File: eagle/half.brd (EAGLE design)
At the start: 138.2 x 89.8 mm, 120 parts, among them J10 AUDIO_JACK_TRRSSMD_RA, J3 AUDIO_JACK_TRRSSMD_RA, J5 AUDIO_JACK_TRRSSMD_RA, J7 AUDIO_JACK_TRRSSMD_RA, J8 AUDIO_JACK_TRRSSMD_RA, J9 AUDIO_JACK_TRRSSMD_RA

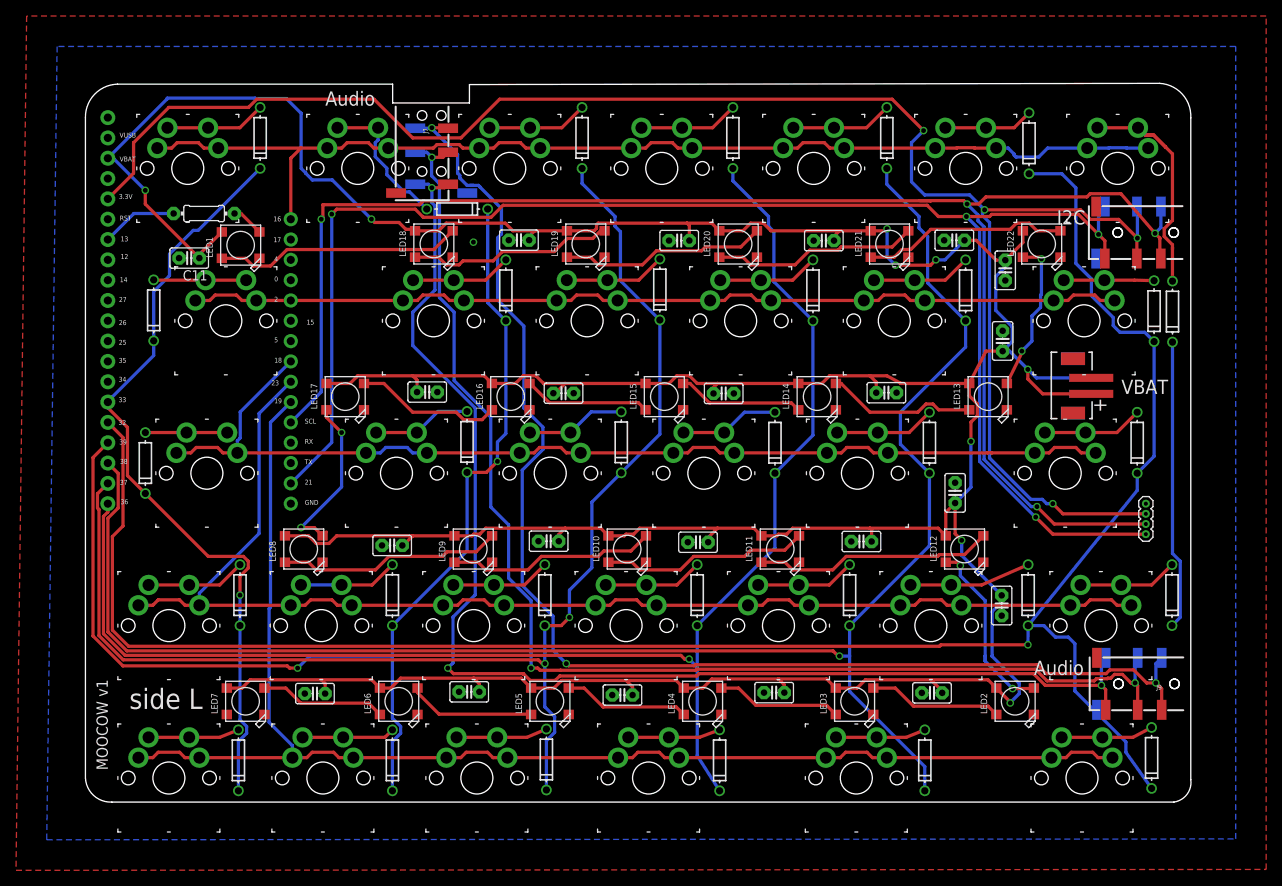
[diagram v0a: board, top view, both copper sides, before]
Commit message: updated PCB
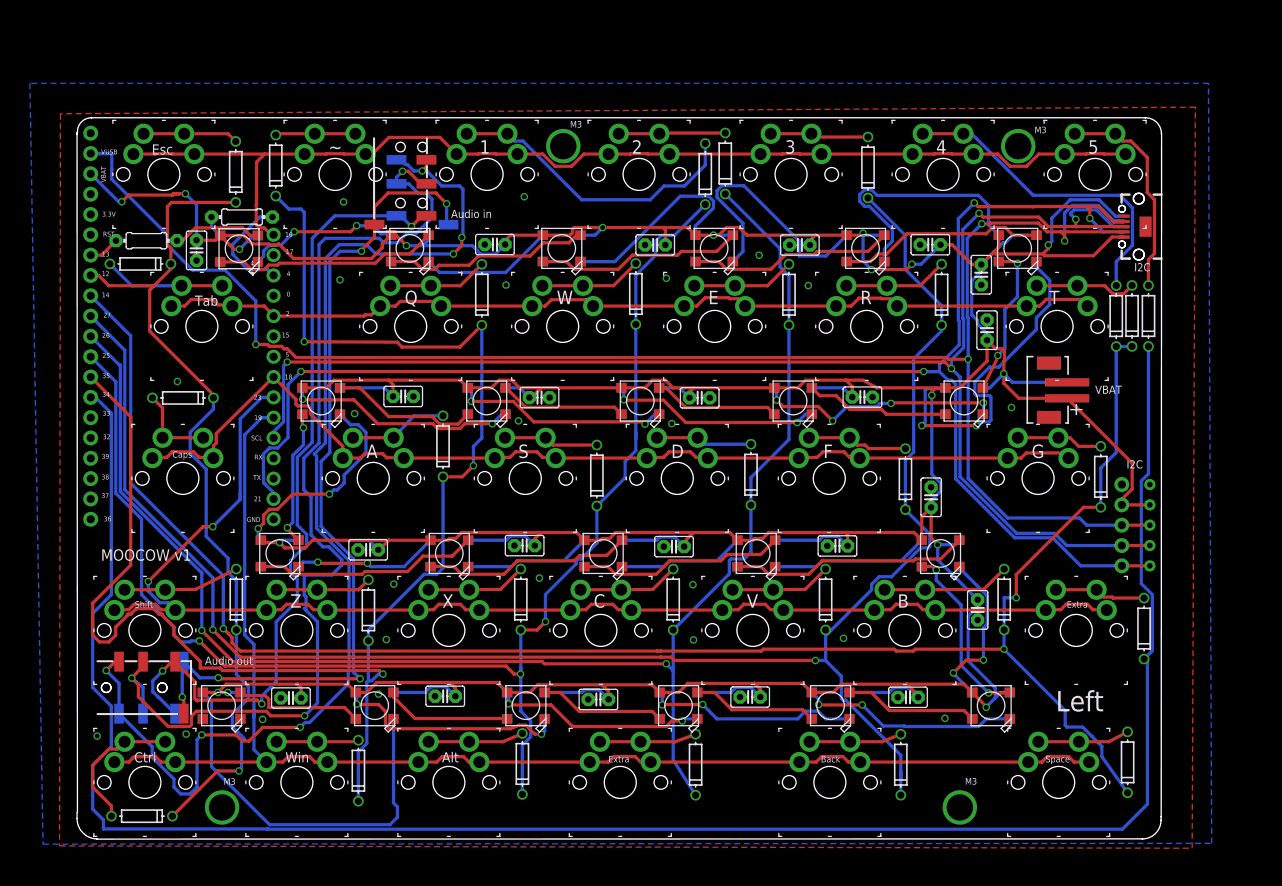
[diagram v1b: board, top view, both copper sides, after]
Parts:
- added J12: (no value), SparkFun-Connectors:1X05_NO_SILK
- added LED23, LED24, LED25, LED26, LED27, LED28, LED29, LED30, LED31, LED32, LED33, LED34, LED35, LED36, LED37, LED38, LED39, LED40, LED41, LED42, LED43, LED44: WS2812B_5050N, adafruit:WS2812B-NARROW
- added R2: 330, adafruit:0204/7
- J2: device SparkFun-Connectors:1X04_1.27MM -> SparkFun-Connectors:1X05_NO_SILK_SMALL
- J3, J5: value AUDIO_JACK_TRRSSMD_RA -> (none); device SparkFun-Connectors:AUDIO_JACK_3.5MM_TRRS_SMD_RA -> SparkFun-Connectors:USB-B-MICRO-SMD-HOLES
- moved J10 136.7 mm to (2.00, 18.9), turned to 180 degrees
- moved J9 136.7 mm to (2.00, 18.9), turned to 0 degrees
- moved D6 24.2 mm to (129.8, 65.4)
- moved D2 23.3 mm to (24.8, 84.2), turned to 270 degrees
- moved D3 16.0 mm to (78.5, 83.1)
- moved D29 13.9 mm to (8.06, 2.85), turned to 0 degrees
- moved D15 9.40 mm to (13.2, 55.1), turned to 0 degrees
- moved R1 7.96 mm to (8.63, 74.8)
- moved D20 6.23 mm to (127.9, 45.3)
- moved D8 6.03 mm to (7.87, 71.9), turned to 0 degrees
- moved D19 5.45 mm to (103.5, 45.0)
- moved D28 5.45 mm to (133.3, 26.3)
- moved D1 5.23 mm to (19.8, 83.4)
- moved J3 5.16 mm to (133.5, 76.5)
- moved J5 5.16 mm to (133.5, 76.5)
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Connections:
- removed net 12: J1.13
- removed net 14: J1.12
- removed net 25: J1.9
- removed net 26: J1.10
- removed net 27: J1.11
- removed net 34: J1.7
- removed net 35: J1.8
- new net 32: J1.5
- new net 33: J1.6
- new net 36: J1.1
- new net 37: J1.2
- new net 38: J1.3
- new net 39: J1.4
- new net N$45: J10.EARTH, J7.EARTH, J8.EARTH, J9.EARTH
- new net N$46: LED30.4-DIN, LED39.2-DOUT
- new net N$47: LED24.4-DIN, LED34.2-DOUT
- new net N$62: LED23.4-DIN, R2.2
- new net N$63: LED24.2-DOUT, LED25.4-DIN
- new net N$64: LED25.2-DOUT, LED26.4-DIN
- new net N$65: LED26.2-DOUT, LED27.4-DIN
- new net N$66: LED27.2-DOUT, LED28.4-DIN
- new net N$67: LED28.2-DOUT, LED29.4-DIN
- new net N$68: LED30.2-DOUT, LED31.4-DIN
- new net N$69: LED31.2-DOUT, LED32.4-DIN
- new net N$70: LED32.2-DOUT, LED33.4-DIN
- new net N$71: LED33.2-DOUT, LED34.4-DIN
- new net N$72: LED35.4-DIN, LED44.2-DOUT
- new net N$73: LED35.2-DOUT, LED36.4-DIN
- new net N$74: LED36.2-DOUT, LED37.4-DIN
- new net N$75: LED37.2-DOUT, LED38.4-DIN
- new net N$76: LED38.2-DOUT, LED39.4-DIN
- new net N$77: LED23.2-DOUT, LED40.4-DIN
- new net N$78: LED40.2-DOUT, LED41.4-DIN
- new net N$79: LED41.2-DOUT, LED42.4-DIN
- new net N$80: LED42.2-DOUT, LED43.4-DIN
- new net N$81: LED43.2-DOUT, LED44.4-DIN
- net +3V3: no longer J2.2, J3.RING1, J5.RING1
- net 4: now also R2.1
- net C1: now also J1.13; no longer J1.6
- net C2: now also J1.8; no longer J1.4
- net C3: now also J1.9; no longer J1.2
- net C4: now also J1.10; no longer J1.1
- net C5: now also J1.11; no longer J1.3
- net C6: now also J1.12; no longer J1.5
- net C7: now also J1.7
- net GND: now also J12.1, J3.GND, J5.GND, LED23.3-GND, LED24.3-GND, LED25.3-GND, LED26.3-GND, LED27.3-GND, LED28.3-GND, LED29.3-GND, LED30.3-GND, LED31.3-GND, LED32.3-GND, LED33.3-GND, LED34.3-GND, LED35.3-GND, LED36.3-GND, LED37.3-GND, LED38.3-GND, LED39.3-GND, LED40.3-GND, LED41.3-GND, LED42.3-GND, LED43.3-GND, LED44.3-GND; no longer J10.EARTH, J3.EARTH, J5.EARTH, J7.EARTH, J8.EARTH, J9.EARTH
- net SCL: now also J12.4, J2.4, J3.D+, J5.D+; no longer J2.3, J3.RING2, J5.RING2
- net SDA: now also J12.5, J2.5, J3.ID, J5.ID; no longer J2.4, J3.TIP, J5.TIP
- net VBAT: now also J12.2, J2.2, J3.VBUS, J5.VBUS, LED23.1-VDD, LED24.1-VDD, LED25.1-VDD, LED26.1-VDD, LED27.1-VDD, LED28.1-VDD, LED29.1-VDD, LED30.1-VDD, LED31.1-VDD, LED32.1-VDD, LED33.1-VDD, LED34.1-VDD, LED35.1-VDD, LED36.1-VDD, LED37.1-VDD, LED38.1-VDD, LED39.1-VDD, LED40.1-VDD, LED41.1-VDD, LED42.1-VDD, LED43.1-VDD, LED44.1-VDD
- net VUSB: now also J12.3, J2.3, J3.D-, J5.D-
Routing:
- net VUSB: track 0.00 -> 215.6 mm, vias 0 -> 4
- net +3V3: track 213.8 -> 0.00 mm, vias 4 -> 0
- net C7: track 36.3 -> 249.4 mm
- net VBAT: track 559.0 -> 710.9 mm, vias 9 -> 17
- net N$45: track 0.00 -> 108.1 mm, vias 0 -> 5
- net N$43: track 160.9 -> 102.8 mm
- net N$67: track 0.00 -> 48.9 mm
- net C2: track 146.4 -> 194.5 mm, vias 2 -> 3
- net N$72: track 0.00 -> 43.0 mm, vias 0 -> 2
- net N$80: track 0.00 -> 33.0 mm
- net N$81: track 0.00 -> 32.2 mm
- net N$73: track 0.00 -> 31.3 mm, vias 0 -> 4
- net N$27: track 11.2 -> 40.8 mm
- net N$66: track 0.00 -> 29.5 mm, vias 0 -> 2
- net N$76: track 0.00 -> 29.1 mm, vias 0 -> 2
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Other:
- board size 138.2 x 89.8 mm -> 135.6 x 90.2 mm
- board text added: """
- board text added: "/"
- board text added: "1"
- board text added: "3"
- board text added: "6"
- board text added: "7"
- board text added: "8"
- board text added: "9"
- board text added: ";"
- board text added: "<"
- board text added: ">"
- board text added: "A"
- board text added: "Alt"
- board text added: "Audio in"
- board text added: "Audio out"
- board text added: "B"
- board text added: "Back"
- board text added: "C"
- board text added: "Caps"
- board text added: "Ctrl"
- board text added: "D"
- board text added: "Del"
- board text added: "Down"
- board text added: "E"
- board text added: "Enter"
- board text added: "Esc"
- board text added: "Extra"
- board text added: "F"
- board text added: "G"
- board text added: "H"
- board text added: "I"
- board text added: "J"
- board text added: "K"
- board text added: "L"
- board text added: "Left"
- board text added: "M"
- board text added: "M3"
- board text added: "N"
- board text added: "NOTE: all switches, LEDs, diodes, resistor and capacitors go on one side of the board; all remaining IO (USB, pogopins and TRRS) go on the opposite side"
- board text added: "NOTE: the alignment pins for the springed male I2C connector will have to be drilled manually"
- board text added: "NOTE: the position of the TRRS ports will hit the alignment pins of the switches. There is no way around this since there isn't enough space between the switches; the workaround will be to trim off the excess pin stickout out of the PCB."
- board text added: "O"
- board text added: "P"
- board text added: "Q"
- board text added: "R"
- board text added: "Right"
- board text added: "S"
- board text added: "Shift"
- board text added: "Space"
- board text added: "T"
- board text added: "Tab"
- board text added: "U"
- board text added: "Up"
- board text added: "V"
- board text added: "W"
- board text added: "Win"
- board text added: "X"
- board text added: "Y"
- board text added: "Z"
- board text added: "[ ]"
- board text added: "top distance from edge of board to switches should be symmetric on top & bottom of board"
- board text added: "~"
- board text removed: "Audio"
- board text removed: "Mounting holes for board"
- board text removed: "Need to check symmetric fit and orientation of ESP32"
- board text removed: "TRRS pads not correct for digikey part"
- board text removed: "larger trace width for VBAT since it will carry LED current?"
- board text removed: "left/right alignment of LEDs (could nudge ESP32 to the right a bit...)"
- board text removed: "location of magnet I2C port?"
- board text removed: "side L"
- board text removed: "side R"
